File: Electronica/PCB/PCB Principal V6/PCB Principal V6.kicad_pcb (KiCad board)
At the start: 2 copper layers, 141.2 x 78.1 mm, 22 parts, among them J1 Conexion Sensores, J10 Conn_01x01, J2 Power Monster, J3 On/Off General, J4 Power Input 2, J5 IDC Placa Botones, J6 Power Input 1, J7 Conn_01x01, J8 Conn_01x01, J9 Conn_01x01, SW1 On/Off Motores

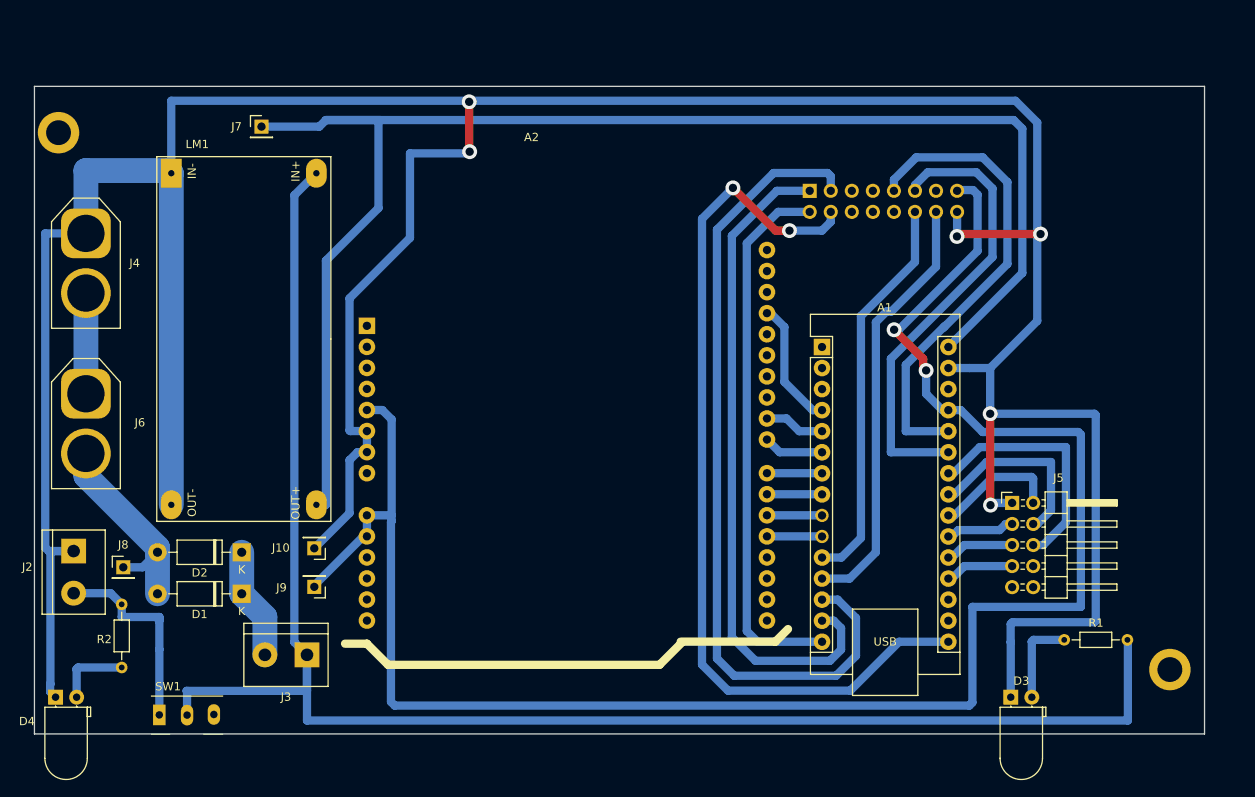
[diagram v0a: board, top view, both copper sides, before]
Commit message: PCB V6 ACTUALIZADA
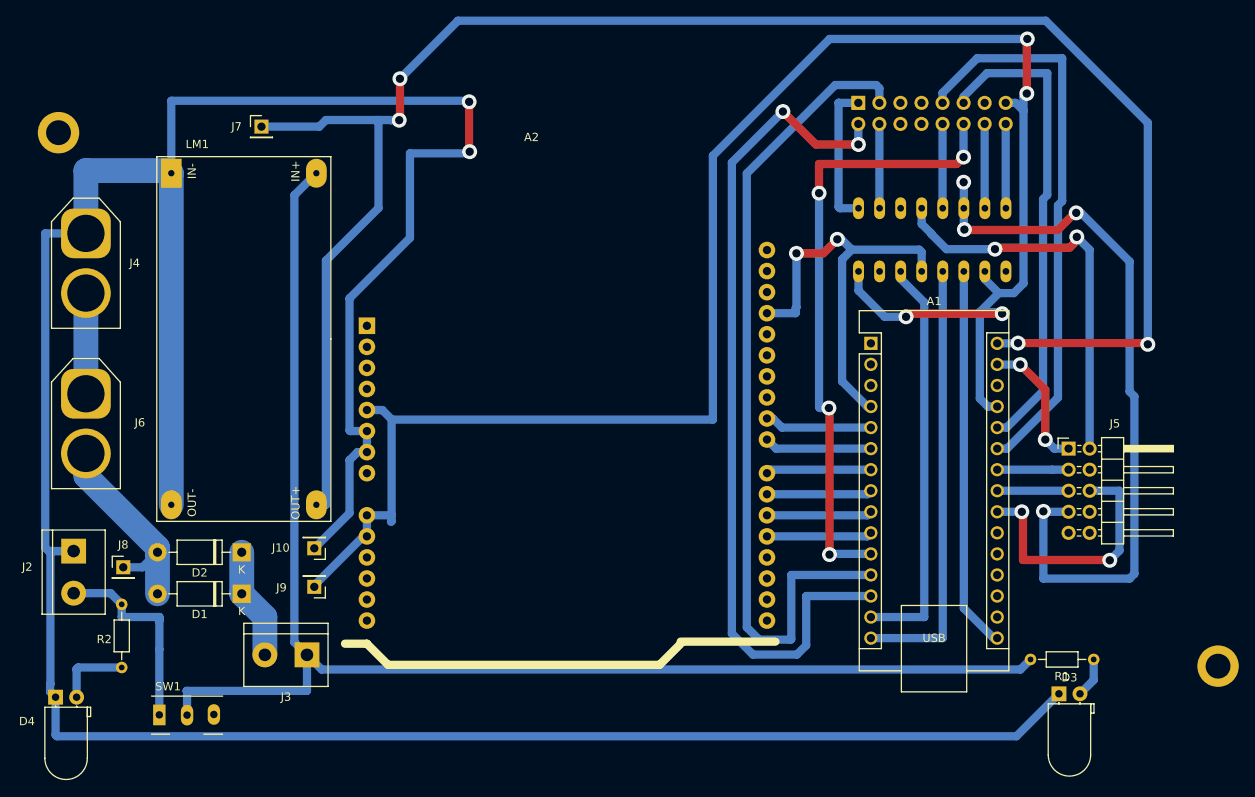
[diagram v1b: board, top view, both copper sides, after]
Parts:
- added U1: 74HC595, 74HC595N_DIP16_:DIP16-2.54-20.32X5.84MM, B.Cu at (190.6, 73.6)
- moved J1 12.1 mm to (181.7, 57.1)
- moved R1 11.9 mm to (202.5, 124.2), turned to 0 degrees
- moved J5 9.45 mm to (207.1, 98.8)
- moved A1 5.91 mm to (183.2, 86.1)
- moved ? 5.82 mm to (225.1, 125.1)
- moved D3 5.82 mm to (205.9, 128.4)
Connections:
- A1 pad 12: TRIG 1 -> ECHO 2
- A1 pad 13: ECHO 2 -> ECHO 3
- A1 pad 14: TRIG 2 -> Data
- A1 pad 15: ECHO 3 -> Latch
- A1 pad 16: TRIG 3 -> Clock
- A1 pad 19: LED1 -> unconnected-(A1-A0-Pad19)
- A1 pad 20: BTN1 -> ECHO 4
- A1 pad 21: BTN2 -> ECHO 5
- A1 pad 22: LED2 -> LED4
- A1 pad 23: LED3 -> BTN1
- A1 pad 24: LED4 -> BTN2
- A1 pad 25: CNY 2 -> CNY 1
- A1 pad 26: CNY 1 -> CNY 2
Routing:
- net TRIG 3: track 108.1 -> 10.2 mm, vias 2 -> 0
- net LED1: track 8.32 -> 89.4 mm, vias 0 -> 4
- net TRIG 2: track 80.2 -> 17.4 mm
- net Latch: track 0.00 -> 52.9 mm
- net Data: track 0.00 -> 49.3 mm
- net Clock: track 0.00 -> 46.2 mm
- net TRIG 1: track 52.2 -> 10.2 mm
- net ECHO 3: track 65.5 -> 103.0 mm, vias 0 -> 2
- net VNano: track 179.4 -> 216.1 mm, vias 0 -> 4
- net LED2: track 15.2 -> 48.9 mm, vias 0 -> 2
- net MOTORES: track 198.4 -> 170.2 mm
- net ECHO 1: track 47.7 -> 75.1 mm, vias 0 -> 4
- net LED3: track 22.7 -> 0.00 mm
- net CNY 1: track 58.0 -> 68.4 mm
- net TRIG 4: track 0.00 -> 10.2 mm
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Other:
- board outline removed
